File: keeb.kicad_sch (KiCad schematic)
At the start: 19 parts, among them SW1 SW_Push, U1 ATmega32U4-A, Y1 16MHz

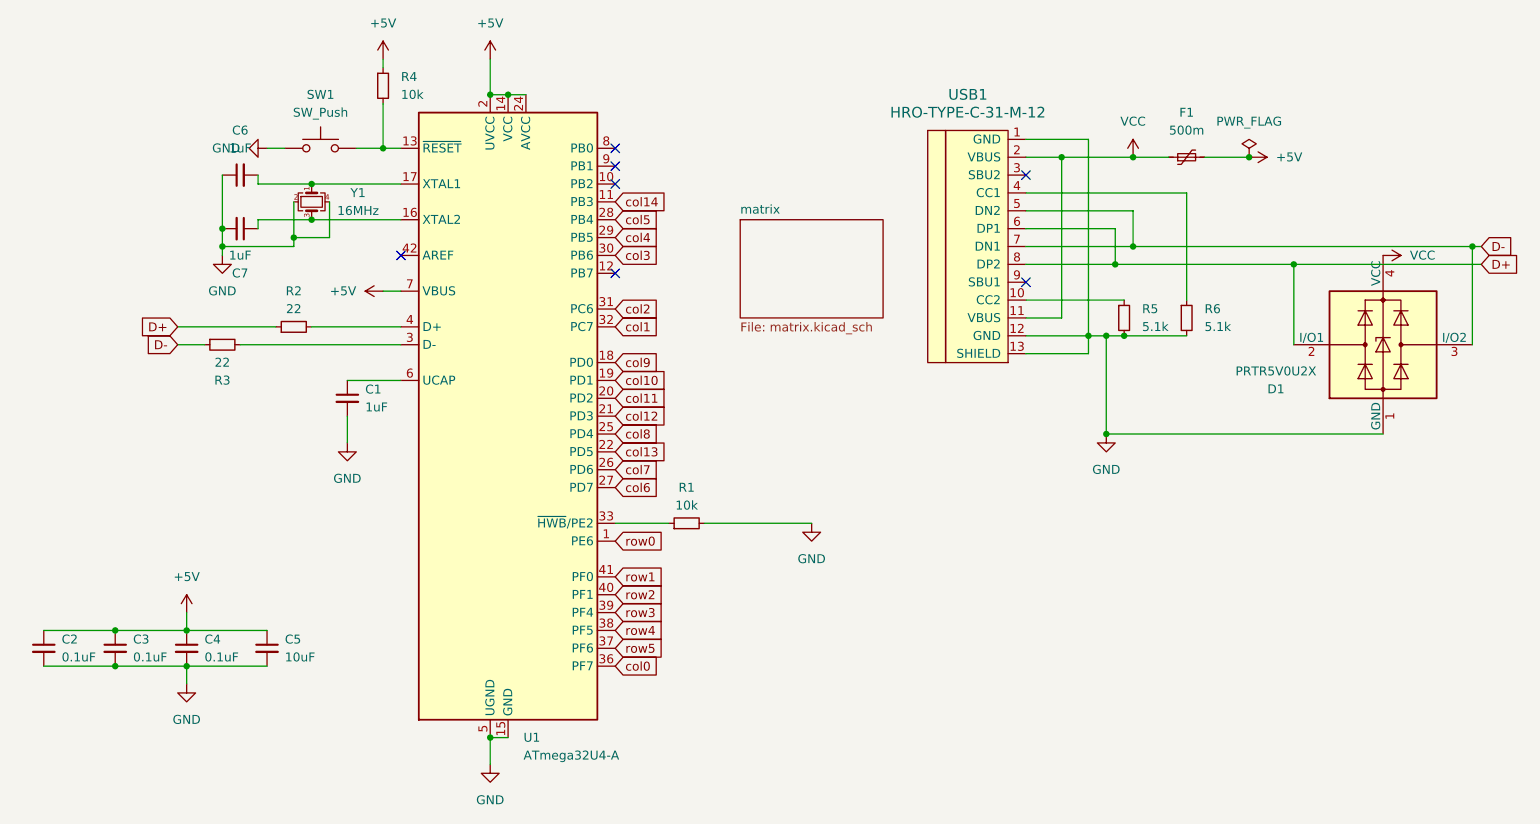
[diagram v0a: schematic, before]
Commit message: fixed mistakes
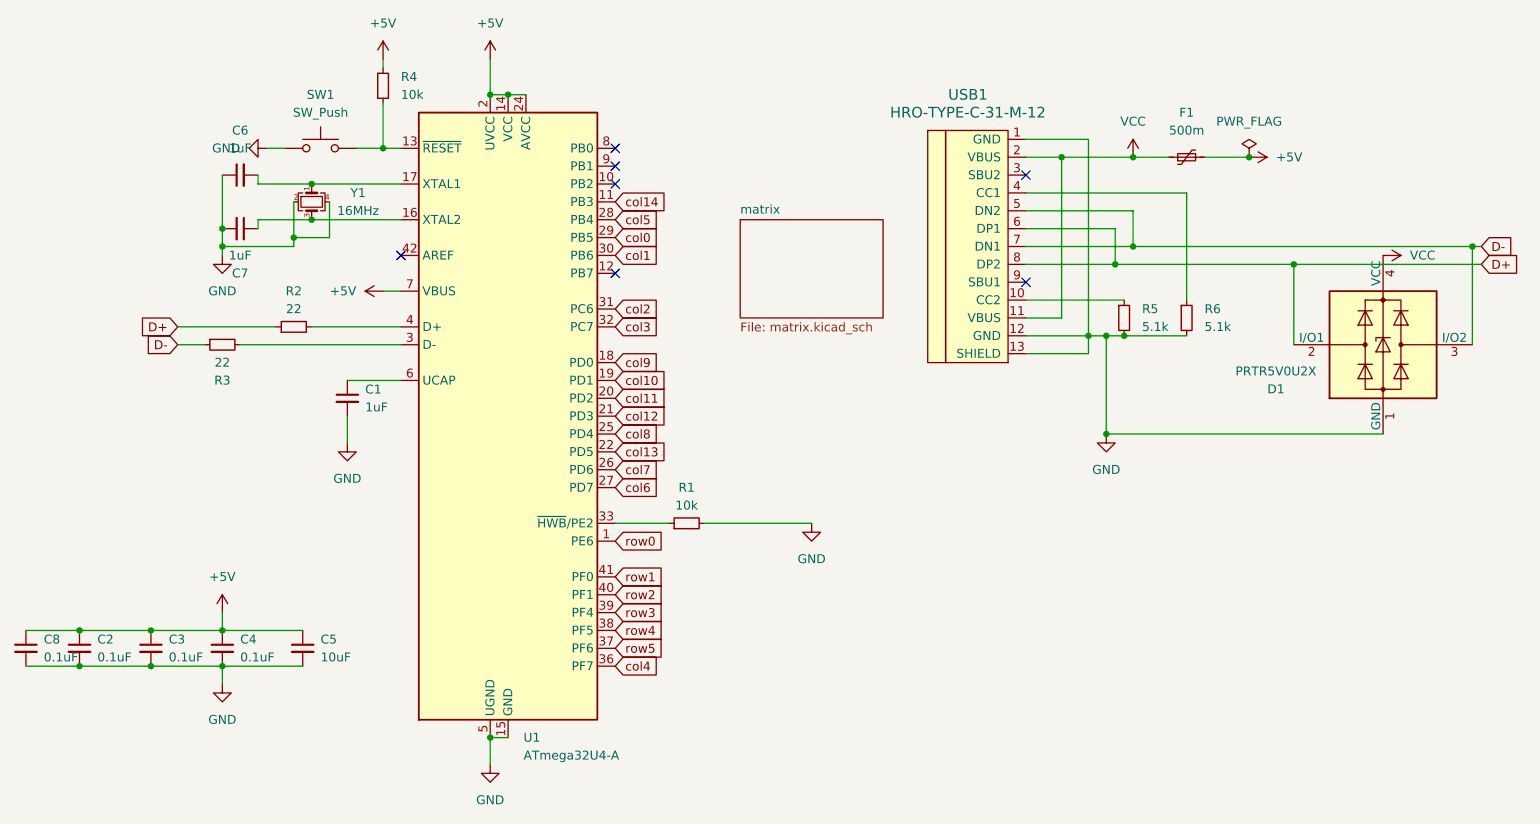
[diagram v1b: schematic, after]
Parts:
- added C8: 0.1uF, Capacitor_SMD:C_0805_2012Metric, symbol Device:C_Small
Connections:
- net +5V: now also C8.1
- net GND: now also C8.2
- net col0: now also U1.29 (PB5); no longer U1.36 (PF7)
- net col1: now also U1.30 (PB6); no longer U1.32 (PC7)
- net col3: now also U1.32 (PC7); no longer U1.30 (PB6)
- net col4: now also U1.36 (PF7); no longer U1.29 (PB5)
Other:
- moved on the sheet: C2, C3, C4, C5
